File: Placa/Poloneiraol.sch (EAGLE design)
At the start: 46 parts, among them X1 MKDSN1,5/4-5,08, X3 MKDSN1,5/2-5,08, X4 MKDSN1,5/2-5,08, X6 MKDSN1,5/10-5,08, X7 MKDSN1,5/4-5,08

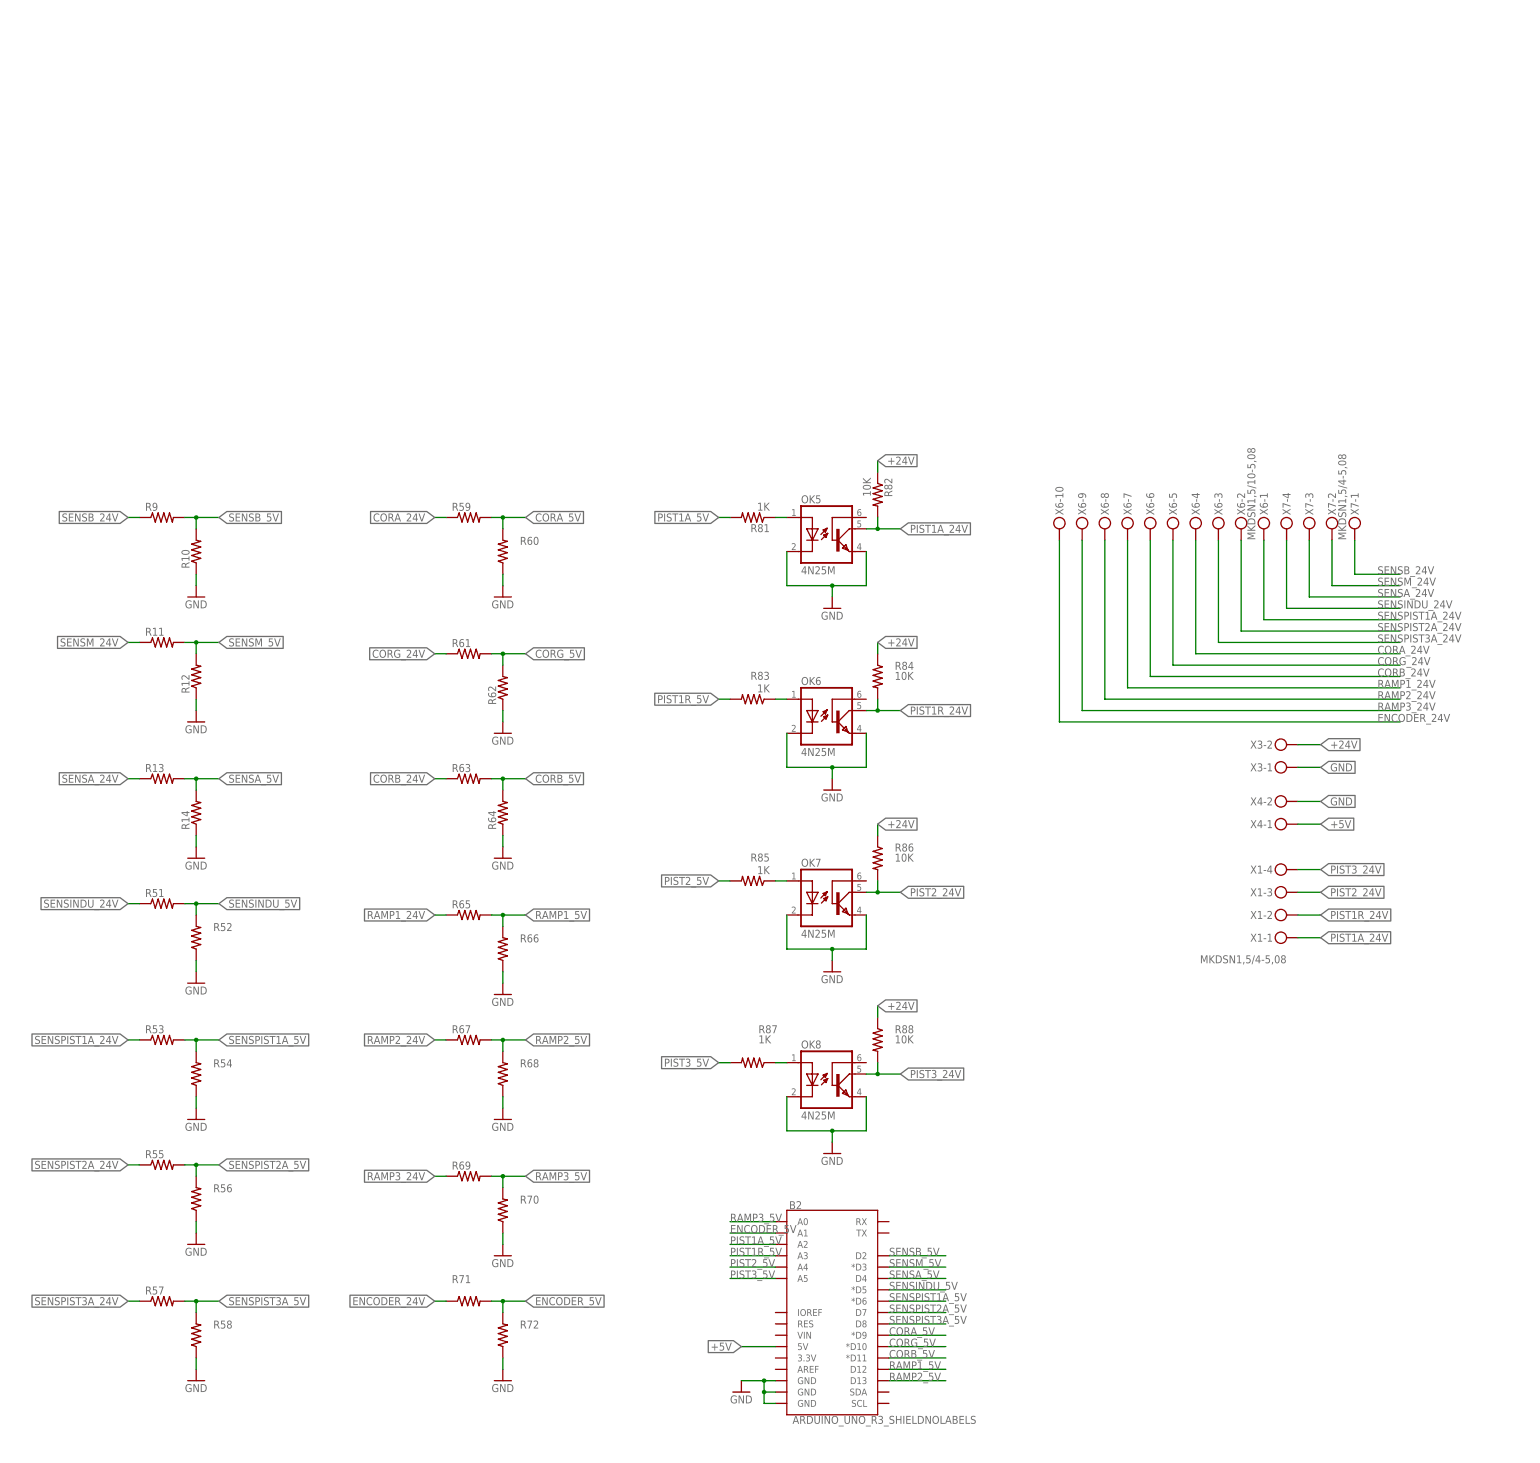
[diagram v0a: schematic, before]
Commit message: 09_11_2018_(2)
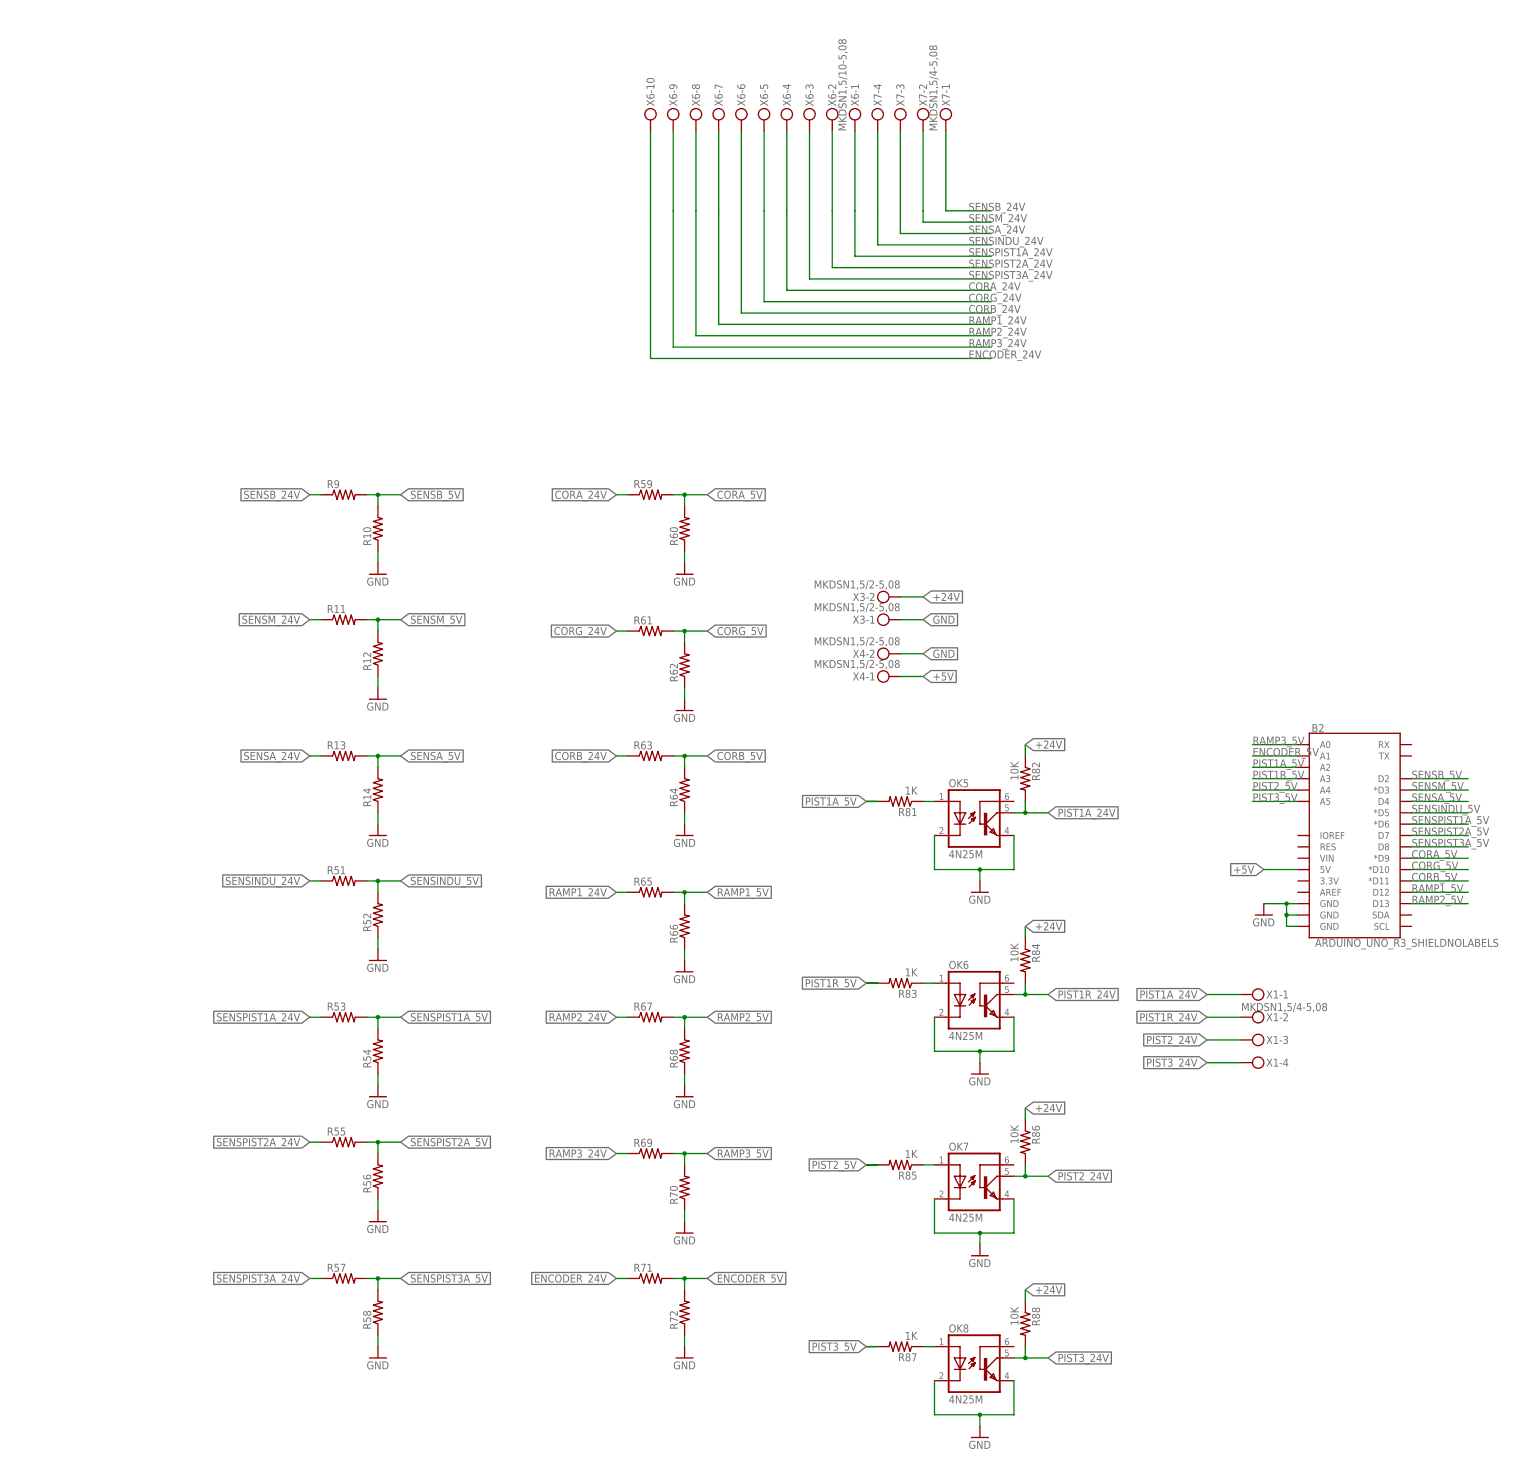
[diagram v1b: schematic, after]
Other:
- moved on the sheet: B2, OK5, OK6, OK7, OK8, R10, R11, R12, R13, R14, R51, R52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
